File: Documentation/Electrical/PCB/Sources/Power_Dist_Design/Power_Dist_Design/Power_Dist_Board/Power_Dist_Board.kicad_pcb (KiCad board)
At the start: 2 copper layers, 175 x 97.5 mm, 47 parts, among them J1 Battery Connector, J2 5V Connector, J3 3.3V Connector, M1 Motor_DC, M2 Motor_DC, M3 Motor_DC, M4 Motor_DC, M5 Motor_DC, M6 Motor_DC, SW1 Emergency Stop, U1 TPS565201, U2 TPS565201

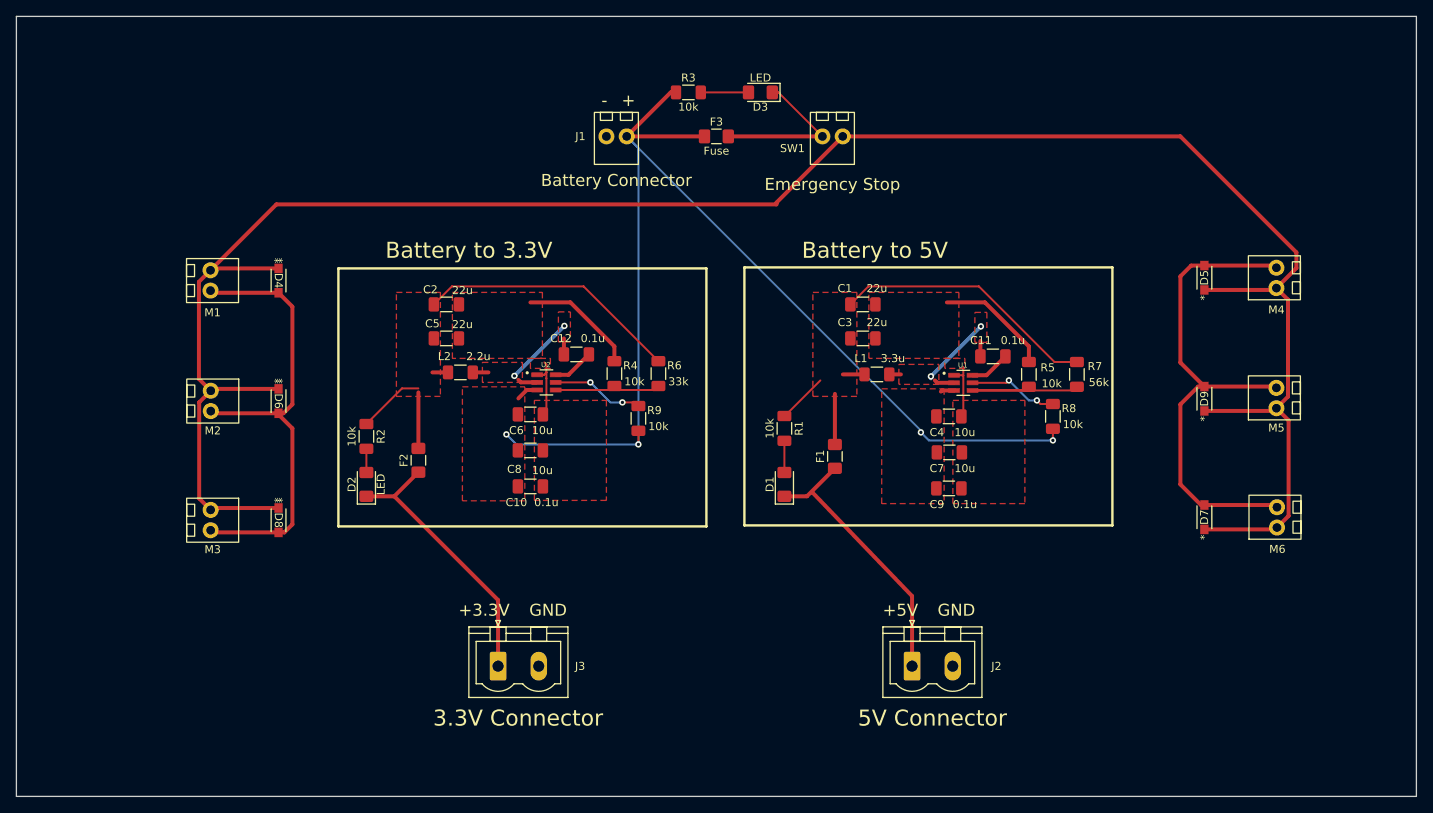
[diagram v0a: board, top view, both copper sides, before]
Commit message: Made further edits to pcb
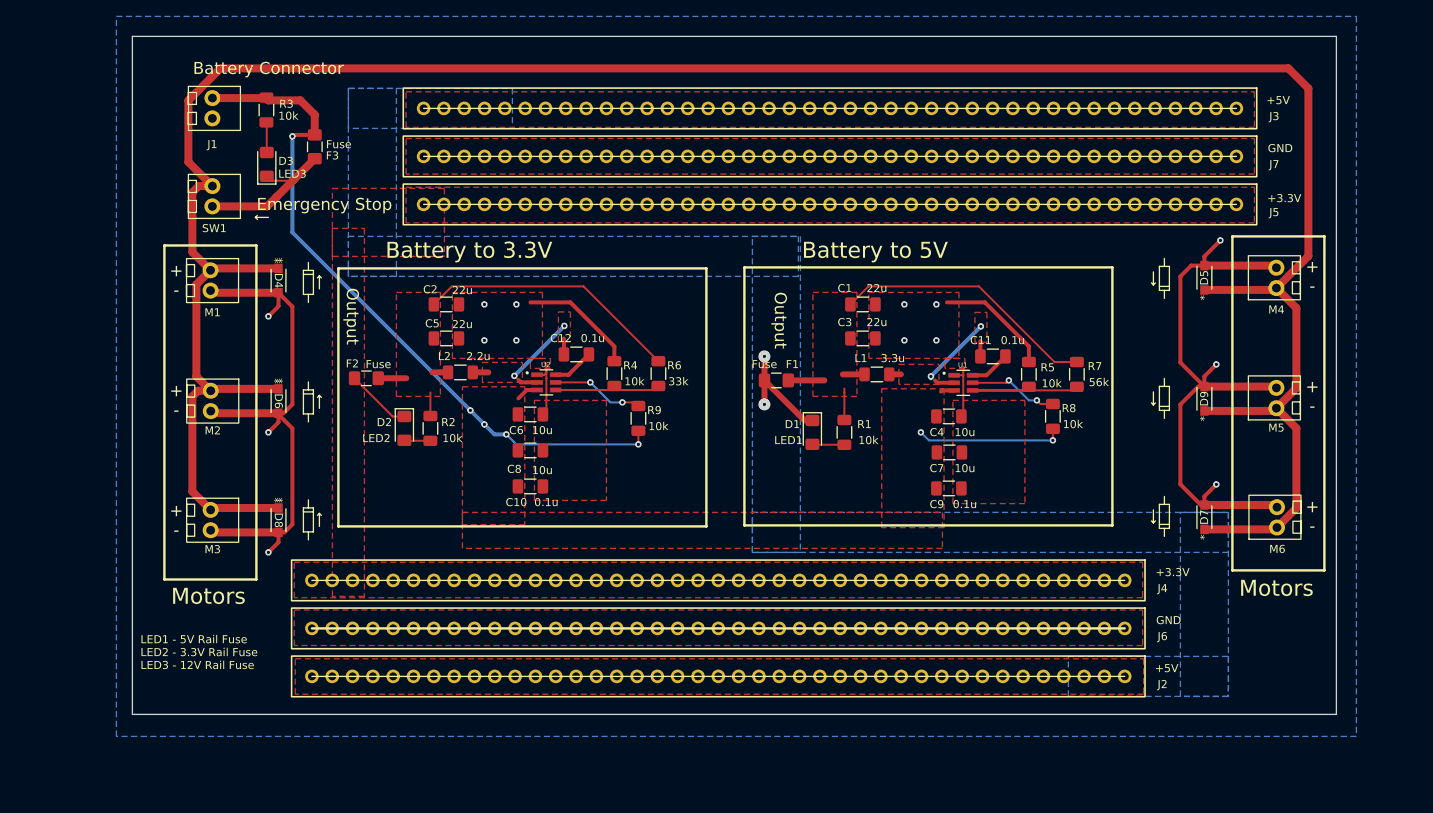
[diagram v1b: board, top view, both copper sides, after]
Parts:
- added J4: +3.3V, Power_Dist:Pwr_Rail_Conn_Custom, F.Cu at (157.8, 88.0)
- added J5: +3.3V, Power_Dist:Pwr_Rail_Conn_Custom, F.Cu at (171.7, 41.0)
- added J6: GND, Power_Dist:Pwr_Rail_Conn_Custom, F.Cu at (157.8, 94.0)
- added J7: GND, Power_Dist:Pwr_Rail_Conn_Custom, F.Cu at (171.7, 35.0)
- D1: value LED -> LED1
- D2: value LED -> LED2
- D3: value LED -> LED3
- J2: value 5V Connector -> +5V; footprint Connector_Phoenix_MSTB:PhoenixContact_MSTBVA_2,5_2-G-5,08_1x02_P5.08mm_Vertical -> Power_Dist:Pwr_Rail_Conn_Custom
- J3: value 3.3V Connector -> +5V; footprint Connector_Phoenix_MSTB:PhoenixContact_MSTBVA_2,5_2-G-5,08_1x02_P5.08mm_Vertical -> Power_Dist:Pwr_Rail_Conn_Custom
- moved J3 82.5 mm to (171.7, 29.0), turned to -90 degrees
- moved SW1 77.9 mm to (92.0, 40.0), turned to -90 degrees
- moved D3 62.4 mm to (98.8, 36.0), turned to 90 degrees
- moved R3 52.8 mm to (98.8, 29.2), turned to -90 degrees
- moved J1 50.6 mm to (92.0, 29.0), turned to -90 degrees
- moved F3 50.2 mm to (104.8, 33.8), turned to -90 degrees
- moved J2 21.7 mm to (157.8, 100.0), turned to -90 degrees
- moved F2 12.1 mm to (111.3, 62.7), turned to 0 degrees
- moved F1 12.0 mm to (162.5, 63.0), turned to 0 degrees
- moved D2 8.46 mm to (116.0, 69.0), turned to -90 degrees
- moved R2 8.06 mm to (119.2, 69.0)
- moved R1 7.52 mm to (171.0, 69.5)
- moved D1 7.38 mm to (167.0, 69.5), turned to -90 degrees
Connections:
- J3 pad 1: +3.3V -> +5V
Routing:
- net +12V: track 272.2 -> 316.2 mm
- net /vin: track 151.1 -> 109.9 mm, vias 4 -> 7
- net +3.3V: track 34.4 -> 8.22 mm
- net +5V: track 34.5 -> 14.1 mm, vias 0 -> 2
- net GND: track 167.8 -> 187.8 mm, vias 0 -> 14
- net /vout2: track 50.2 -> 41.3 mm
- net /vout1: track 48.5 -> 44.3 mm
- net Net-(D3-Pad2): track 5.96 -> 3.78 mm
- net Net-(D3-Pad1): track 20.3 -> 18.7 mm
- added copper zone on F.Cu, net +3.3V
- added copper zone on B.Cu, net +5V
- added copper zone on F.Cu, net +5V
- added copper zone on B.Cu, net GND
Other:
- board size 175 x 97.5 mm -> 150.5 x 84.8 mm
- board text added: "+ -"
- board text added: "LED1 - 5V Rail Fuse LED2 - 3.3V Rail Fuse LED3 - 12V Rail Fuse"
- board text added: "Motors"
- board text added: "Output"
- board text removed: "+"
- board text removed: "+3.3V"
- board text removed: "+5V"
- board text removed: "-"
- board text removed: "GND"
